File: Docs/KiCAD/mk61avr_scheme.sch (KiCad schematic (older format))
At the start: 44 parts, among them IC1 ATMEGA8-P, K1 CONN_3, P1 CONN_4, P2 CONN_5X2, SW1 ON/OFF, SW10 2, SW11 X, SW12 RET, SW13 SAVE, SW14 3, SW15 3, SW16 SUB, SW17 LOAD, SW18 4, SW19 XY, SW2 0, SW20 STORE, SW21 5, SW22 ,, SW23 STEP>, SW24 6, SW25 /-/, SW26 LOAD, SW27 7, SW28 POW, SW29 <STEP, SW3 +, SW30 8, SW31 Cx, SW32 K, SW33 9, SW34 Bx, SW35 F, SW36 SW_PUSH, SW4 S/S, SW5 LFT, SW6 1, SW7 -, SW8 GOTO, SW9 RGT

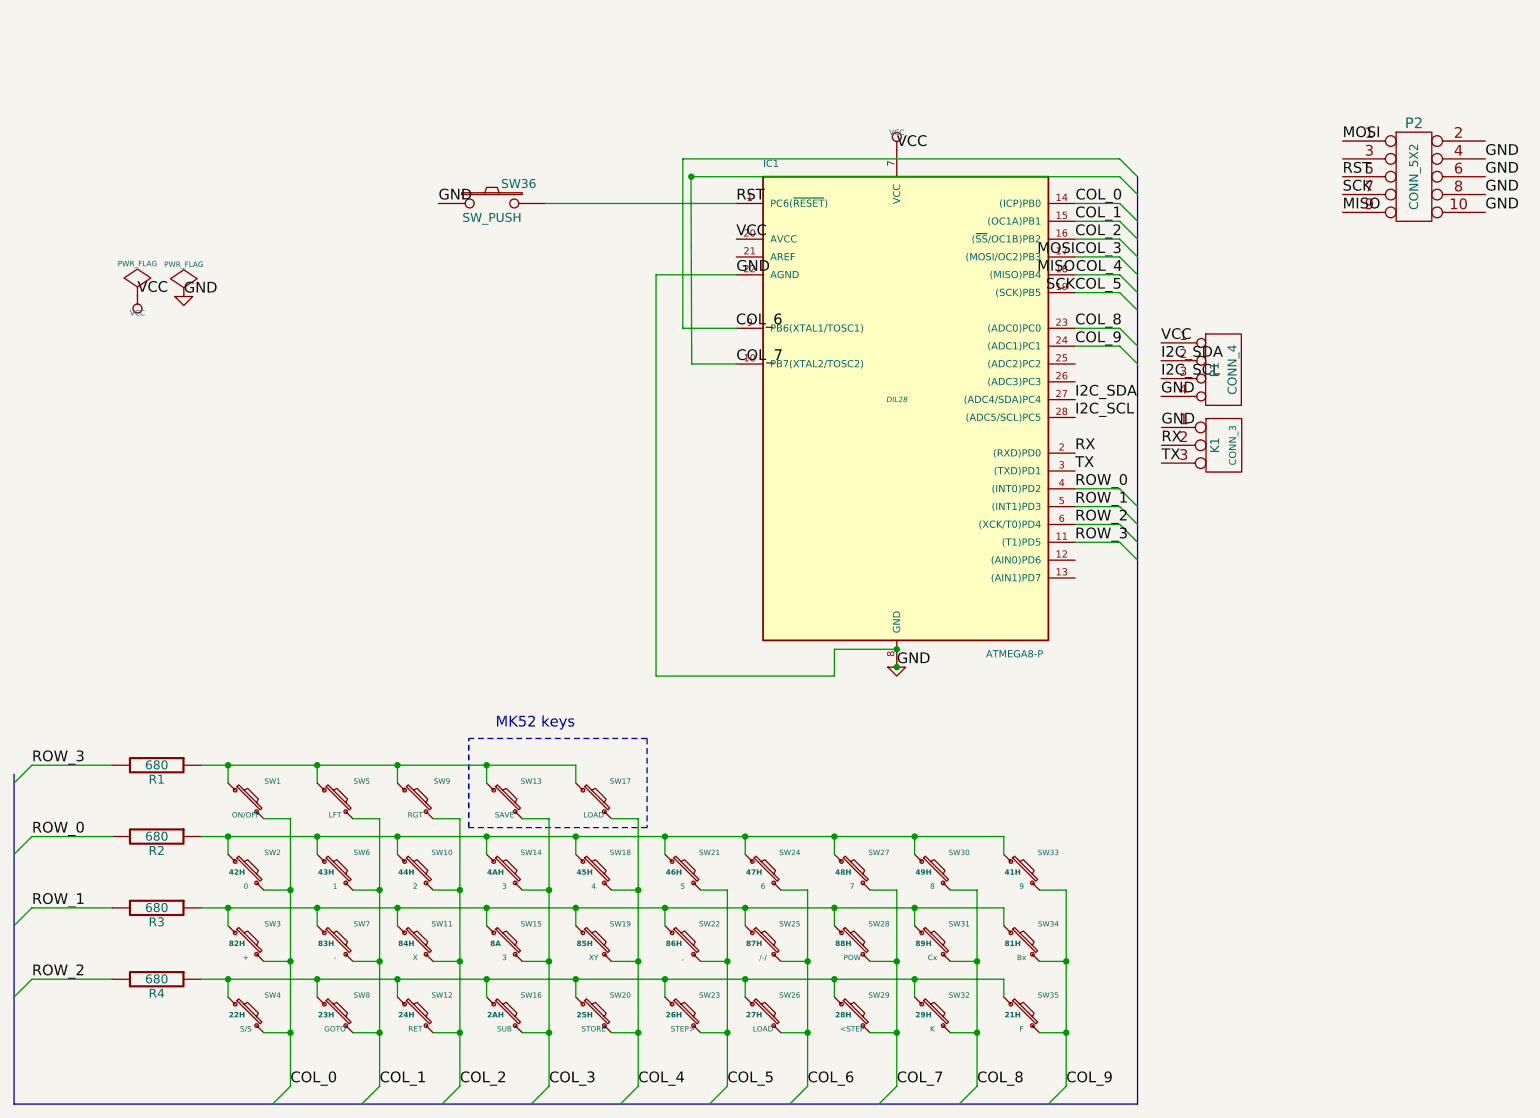
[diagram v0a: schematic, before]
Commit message: KiCAD: обновил схему от Алексея
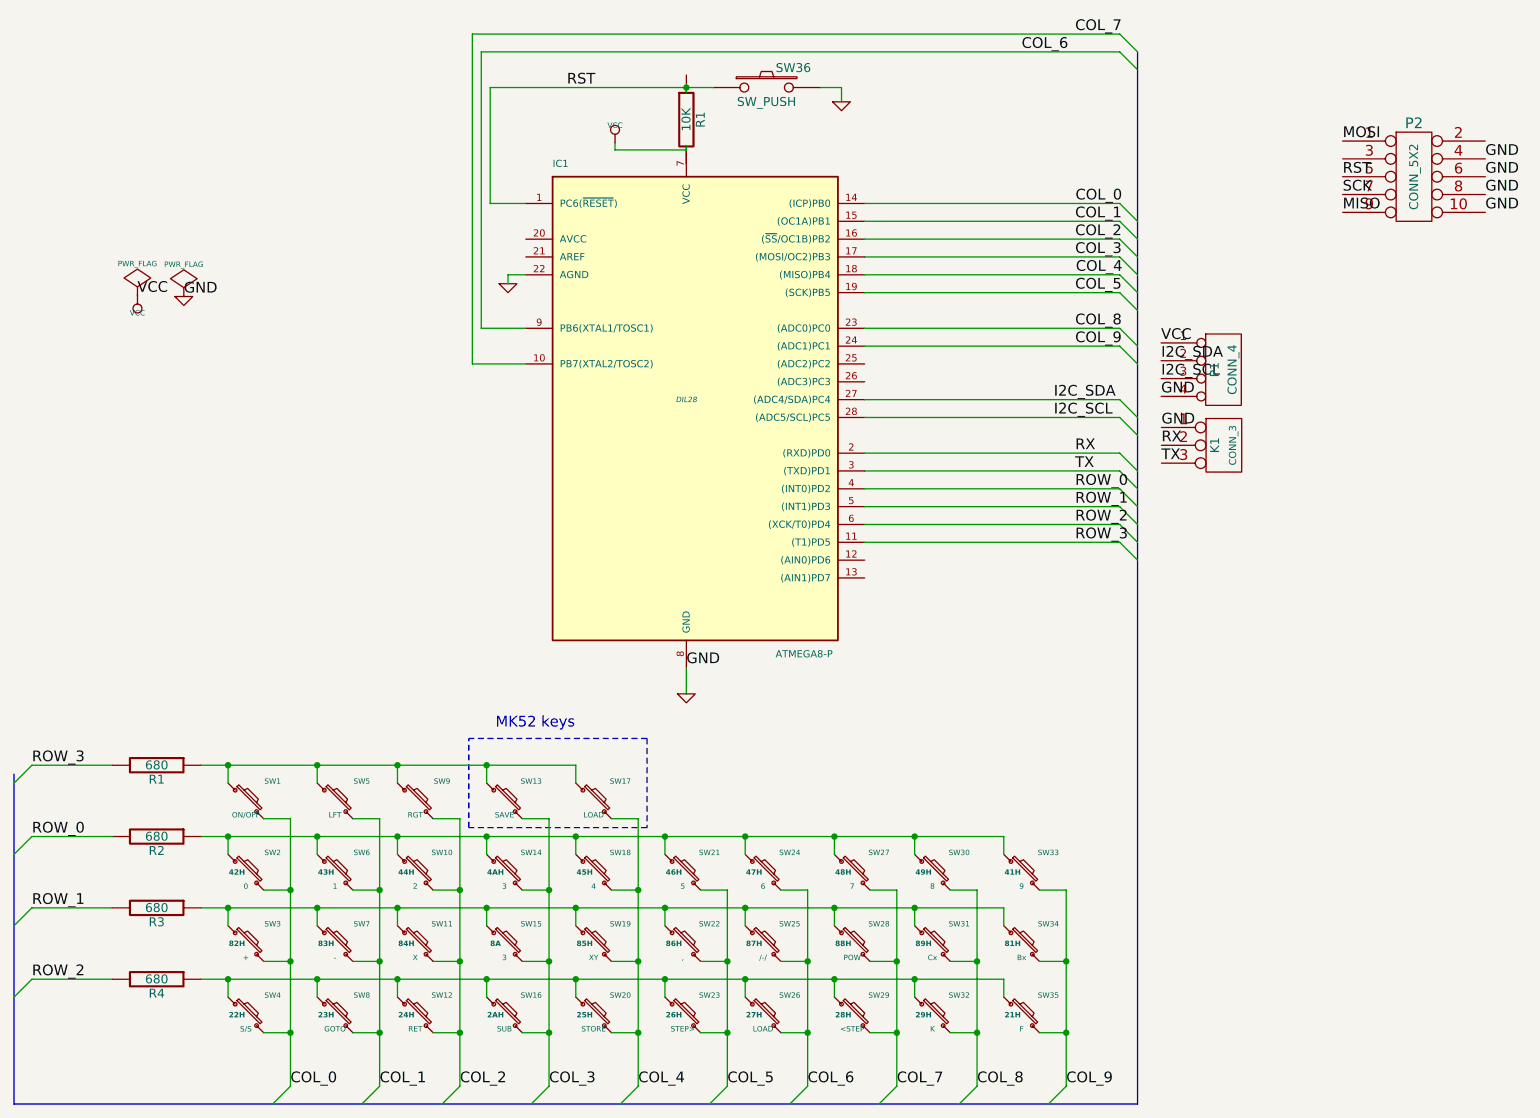
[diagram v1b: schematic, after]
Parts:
- added R1: 10K, symbol R
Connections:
- net COL_3: no longer P2.1
- net COL_4: no longer P2.9
- net COL_5: no longer P2.7
- net GND: now also SW36.2; no longer SW36.1
- net RST: now also SW36.1; no longer SW36.2
- net VCC: no longer IC1.20 (AVCC), IC1.7 (VCC)
- new net MISO: P2.9
- new net MOSI: P2.1
- new net SCK: P2.7
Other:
- moved on the sheet: IC1, SW36
